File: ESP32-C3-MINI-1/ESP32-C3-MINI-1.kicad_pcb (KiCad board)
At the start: 2 copper layers, 20.3 x 31.1 mm, 25 parts, among them J1 ESPProg-UART, J2 USB2.0_C, SW1 RESET, SW2 BOOT, U1 ESP32-C3-MINI-1, U2 AMS1117-3.3

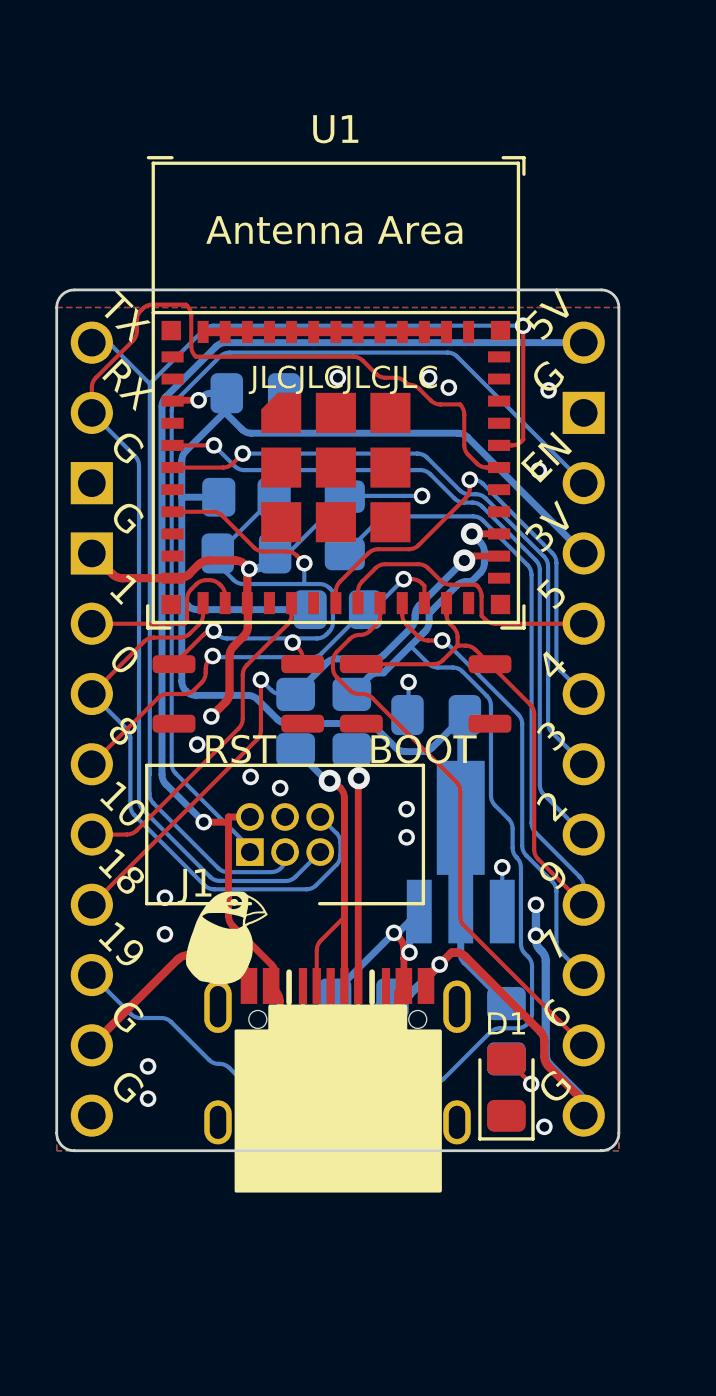
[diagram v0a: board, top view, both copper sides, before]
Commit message: v1.2.0
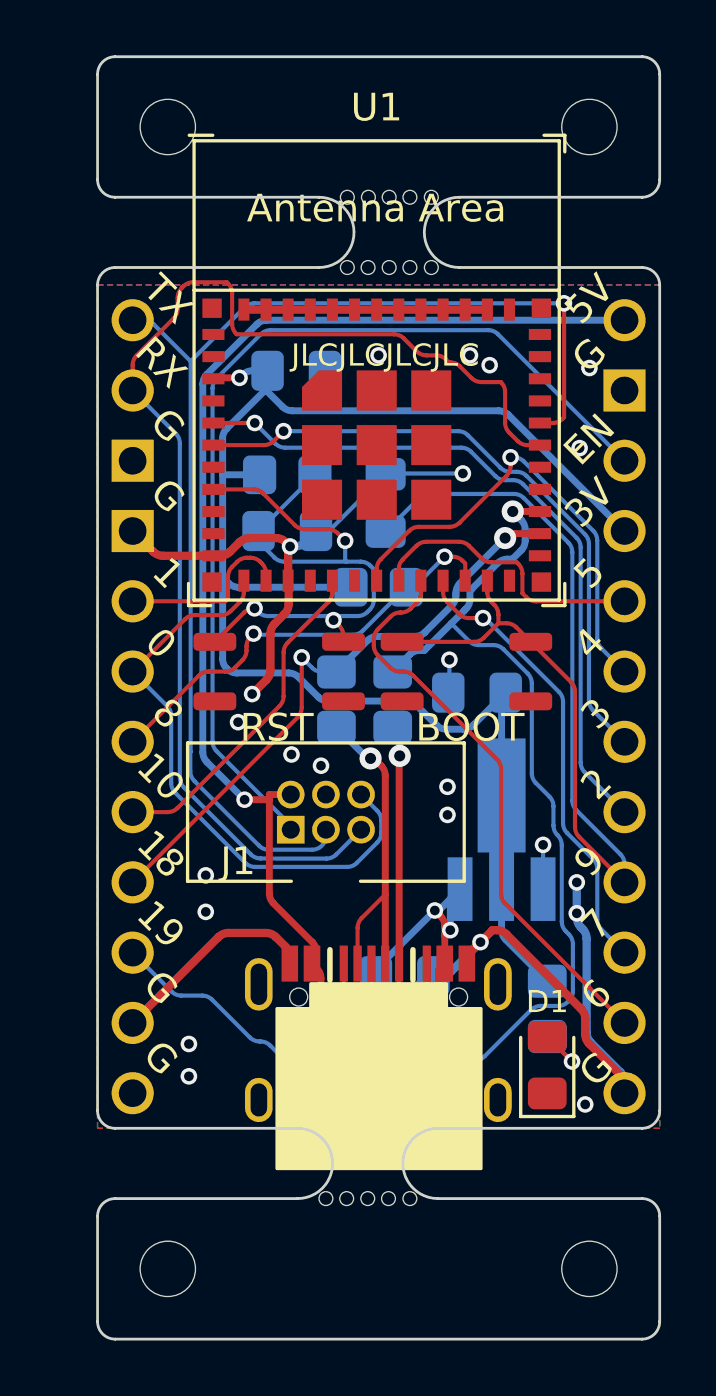
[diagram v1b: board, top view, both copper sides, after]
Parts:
- removed the G*** at (94.9, 106.8)
- added REF**: StencilHole2mm, $74th:StencilHole2mm, F.Cu at (92.9, 118.6)
- added REF**: StencilHole2mm, $74th:StencilHole2mm, F.Cu at (108.2, 77.3)
- added REF**: StencilHole2mm, $74th:StencilHole2mm, F.Cu at (92.9, 77.3)
- added REF**: StencilHole2mm, $74th:StencilHole2mm, F.Cu at (108.2, 118.6)
- added mouse-bite-3mm-slot: VAL**, $74th:mouse-bite-2.54mm-slot, F.Cu at (100.9, 81.1)
- added mouse-bite-3mm-slot: VAL**, $74th:mouse-bite-2.54mm-slot, F.Cu at (100.1, 114.8)
- moved REF** 1.91 mm to (96.7, 106.6)
- moved C2 1.68 mm to (100.8, 90.9)
- moved C1 1.68 mm to (97.6, 86.1)
- moved C4 1.68 mm to (104.1, 97.7)
- moved C5 1.68 mm to (101.5, 108.0)
- moved CH1 1.68 mm to (91.6, 98.2)
- moved CH2 1.68 mm to (109.4, 99.5)
- moved D1 1.68 mm to (106.6, 111.2)
- moved J1 1.68 mm to (98.6, 102.1)
- moved J2 1.68 mm to (100.5, 112.4)
- moved R1 1.68 mm to (97.2, 89.9)
- moved R2 1.68 mm to (100.5, 93.9)
- moved R3 1.68 mm to (101.0, 98.0)
- moved R4 1.68 mm to (99.0, 98.0)
- moved R5 1.68 mm to (106.6, 109.2)
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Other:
- board size 20.3 x 31.1 mm -> 20.3 x 46.4 mm
